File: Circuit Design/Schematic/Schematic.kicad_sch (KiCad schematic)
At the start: 18 parts, among them U1 ESP32-WROOM-32

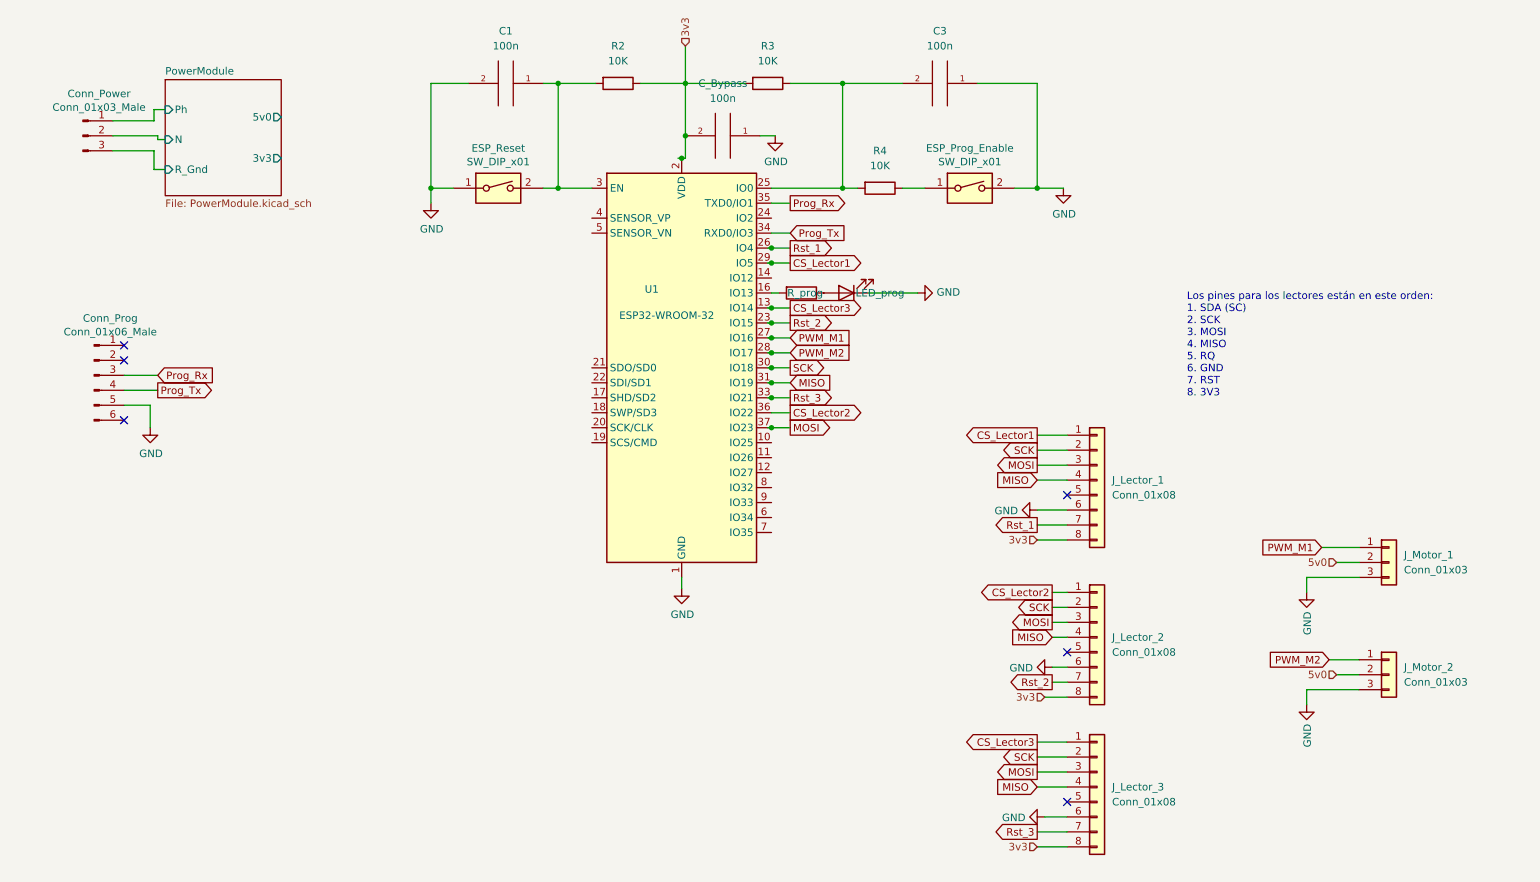
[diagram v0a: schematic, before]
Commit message: Add files via upload
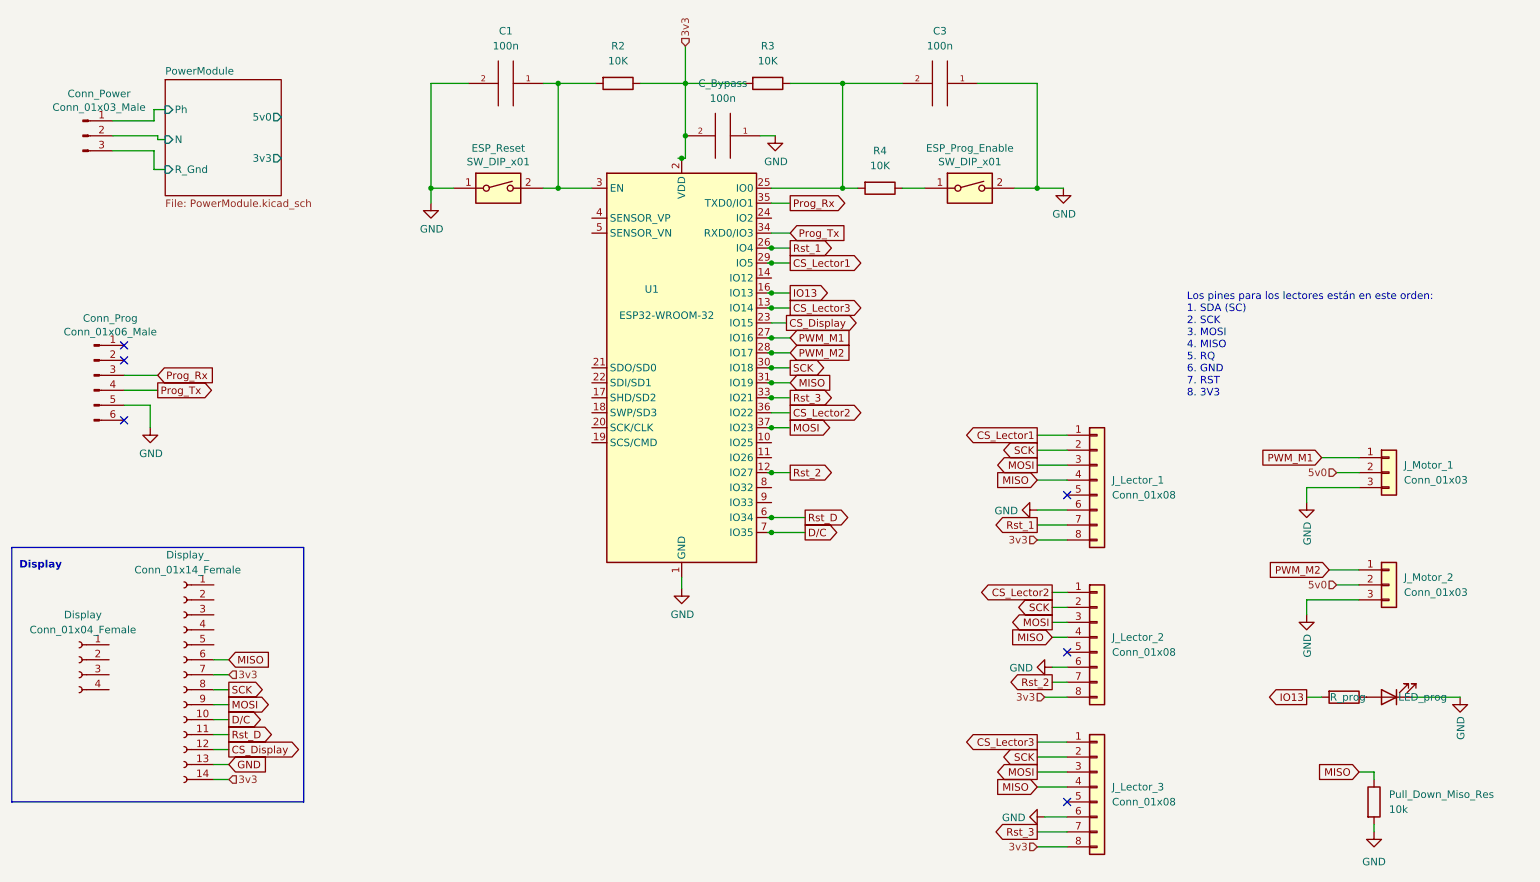
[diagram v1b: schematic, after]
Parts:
- added Display: Conn_01x04_Female, Connector_PinSocket_2.54mm:PinSocket_1x04_P2.54mm_Vertical, symbol Connector:Conn_01x04_Female
- added Display_: Conn_01x14_Female, Connector_PinSocket_2.54mm:PinSocket_1x14_P2.54mm_Vertical, symbol Connector:Conn_01x14_Female
- added Pull_Down_Miso_Res: 10k, symbol Device:R
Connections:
- net 3v3: now also Display_.14 (Pin_14), Display_.7 (Pin_7)
- net GND: now also Display_.13 (Pin_13), Pull_Down_Miso_Res.2
- net MISO: now also Display_.6 (Pin_6), Pull_Down_Miso_Res.1
- net MOSI: now also Display_.9 (Pin_9)
- net Rst_2: now also U1.12 (IO27); no longer U1.23 (IO15)
- net SCK: now also Display_.8 (Pin_8)
- net IO13: now reaches R_prog.2, U1.16 (IO13)
- net Rst_D: now reaches U1.6 (IO34)
- net Rst_D: now also Display_.11 (Pin_11)
- net D/C: now reaches U1.7 (IO35)
- net D/C: now also Display_.10 (Pin_10)
- new net CS_Display: Display_.12 (Pin_12), U1.23 (IO15)
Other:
- note added: "Display"
- moved on the sheet: J_Motor_1, J_Motor_2, LED_prog, R_prog
